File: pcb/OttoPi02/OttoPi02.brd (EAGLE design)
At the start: 55.9 x 64.4 mm, 22 parts

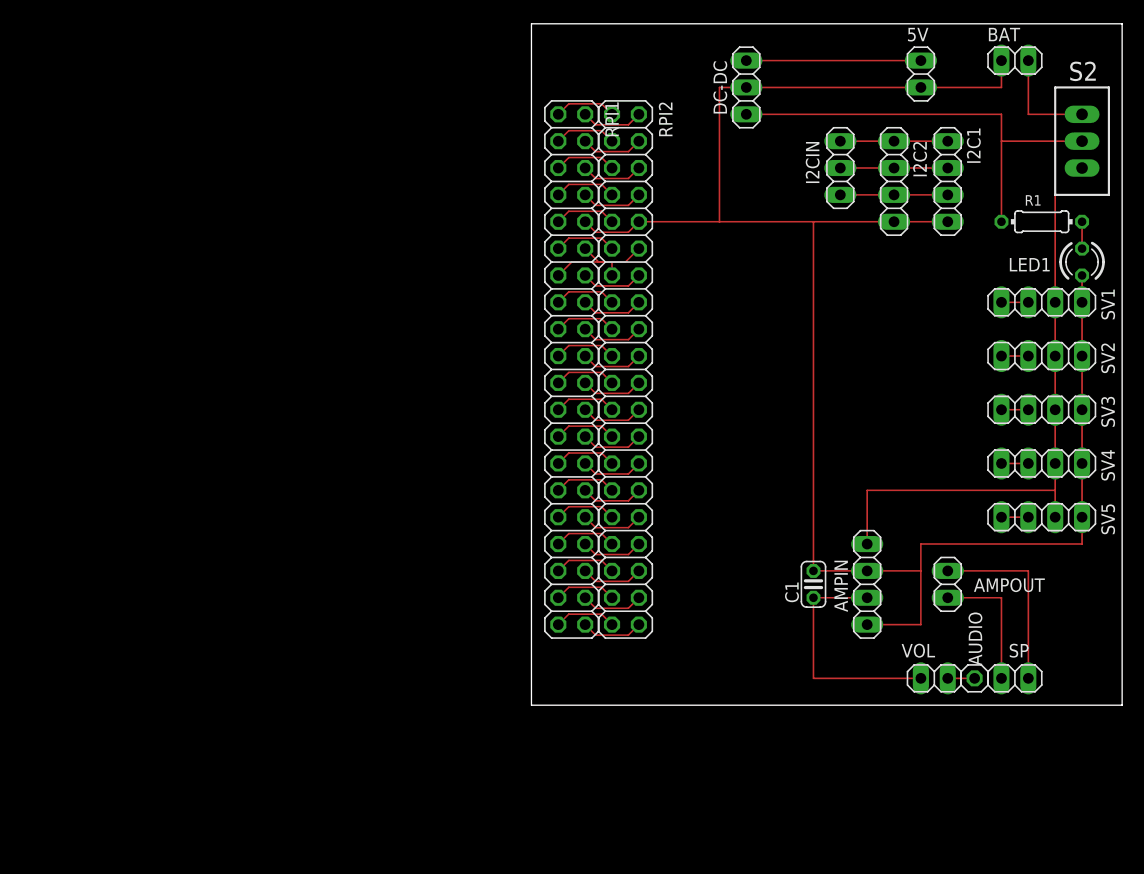
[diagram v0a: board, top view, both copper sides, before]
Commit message: update pcb
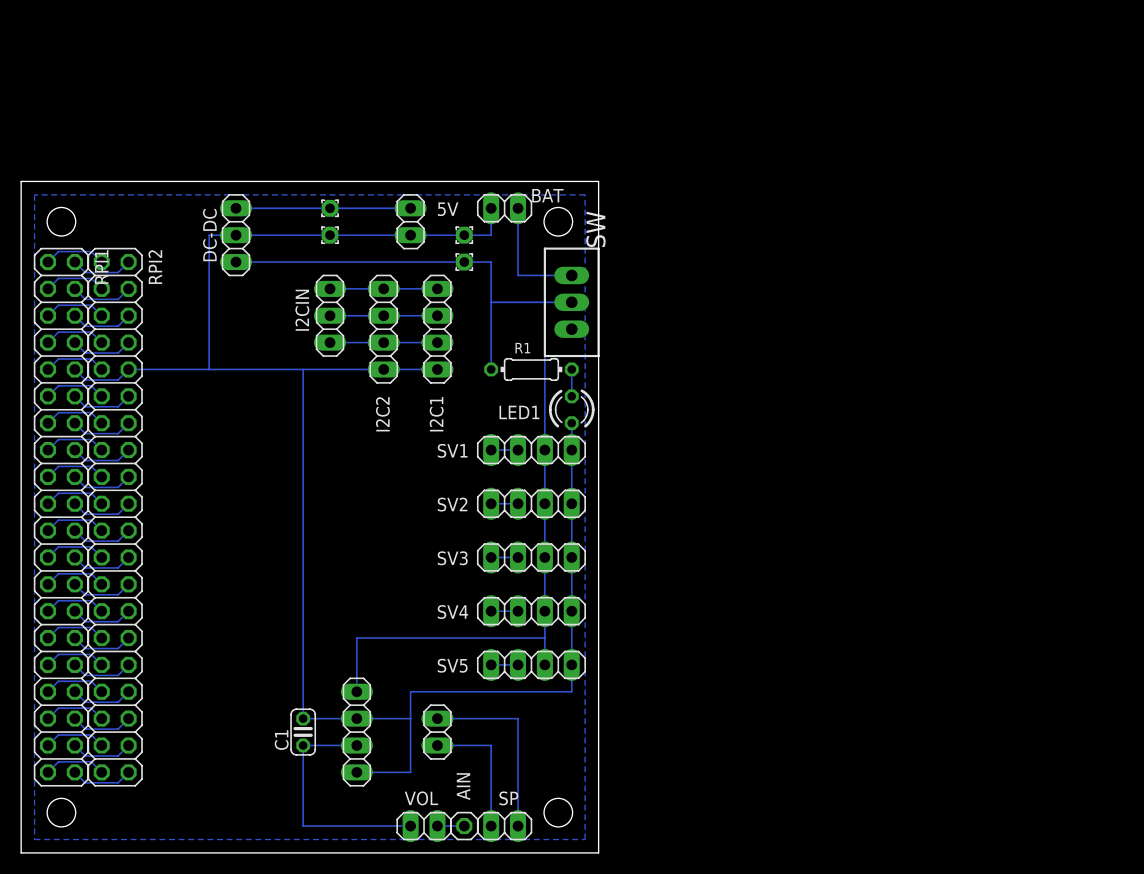
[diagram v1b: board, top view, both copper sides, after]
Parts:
- removed AUDIO: (no value), pinhead:1X01
- removed S2: TL36PO, switch:TL3XPO
- added 5V_A, BAT_B, GND_A, GND_B: (no value), wirepad:1,6/0,9
- added AIN: (no value), pinhead:1X01
- added SW: TL36PO, switch:TL3XPO
- moved AMPOUT 50.2 mm to (40.6, 14.0)
- moved C1 50.2 mm to (27.9, 14.0)
- moved I2C1 50.2 mm to (40.6, 52.1)
- moved R1 50.2 mm to (49.5, 48.3)
- moved RPI1 50.2 mm to (5.08, 34.3)
- moved RPI2 50.2 mm to (10.2, 34.3)
- moved SV1 50.2 mm to (49.5, 40.6)
- moved SV2 50.2 mm to (49.5, 35.6)
- moved SV3 50.2 mm to (49.5, 30.5)
- moved SV4 50.2 mm to (49.5, 25.4)
- moved SV5 50.2 mm to (49.5, 20.3)
- moved 5V 50.2 mm to (38.1, 62.2)
- moved AMPIN 50.2 mm to (33.0, 14.0)
- moved BAT 50.2 mm to (47.0, 63.5)
- moved SP 50.2 mm to (47.0, 5.08)
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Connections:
- removed net N$18: RPI1.5, RPI2.5
- net GND: now also GND_A.1, GND_B.1, RPI1.5, RPI2.5
- net N$13: now also BAT_B.1, SW.2; no longer S2.2
- net N$14: now also AIN.1; no longer AUDIO.1
- net N$5: now also 5V_A.1
- net N$7: now also SW.1; no longer S2.1
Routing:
- net GND: track 173.5 -> 179.4 mm
- net N$18: track 5.90 -> 0.00 mm
- net N$7: track 10.2 -> 11.4 mm
- net N$13: track 100.3 -> 99.1 mm
- net N$22: track 6.88 -> 5.90 mm
- added copper zone on layer 16, net GND
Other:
- board size 55.9 x 64.4 mm -> 54.6 x 63.5 mm

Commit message: update
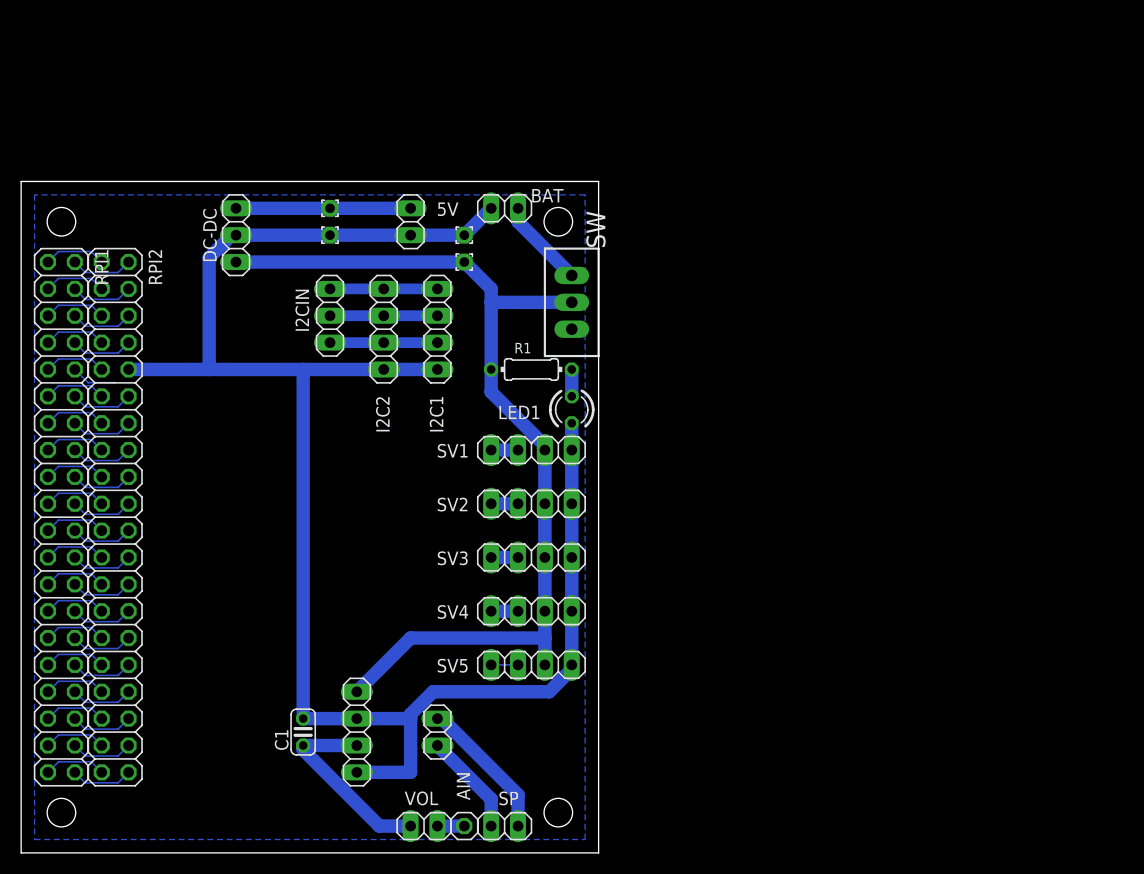
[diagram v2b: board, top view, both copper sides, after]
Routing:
- net N$13: track 99.1 -> 90.4 mm
- net GND: track 179.4 -> 172.7 mm
- net N$12: track 17.8 -> 13.6 mm
- net N$8: track 22.9 -> 18.6 mm
- net N$7: track 11.4 -> 8.45 mm
- net N$4: track 12.7 -> 9.72 mm
